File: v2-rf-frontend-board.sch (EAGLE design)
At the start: 150 parts, among them J1 1.27MM-SWD-CONNECTOR, J2 CON_SMA-ENDFIRE_EMERSON_EMERS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, J3 ROCKETNET-CONNECTOR-16M, J4 ZX62D-B-5P8, J5 BREAKOUT, J7 CON_HIROSE_DM3D(MICROSD), Q1 NTR4101P, T1 ALT4532, T2 ALT4532, U1 MAX2769, U2 STM32F4V_100PIN_GPSBOARD, U3 KSZ8081, U4 7Q-16.368MBG-T, U5 XC2401A8167R-G, U6 MAX8510EXK29+T, U7 MAX8510EXK29+T, U8 LMZ12001, X1 25 MHz

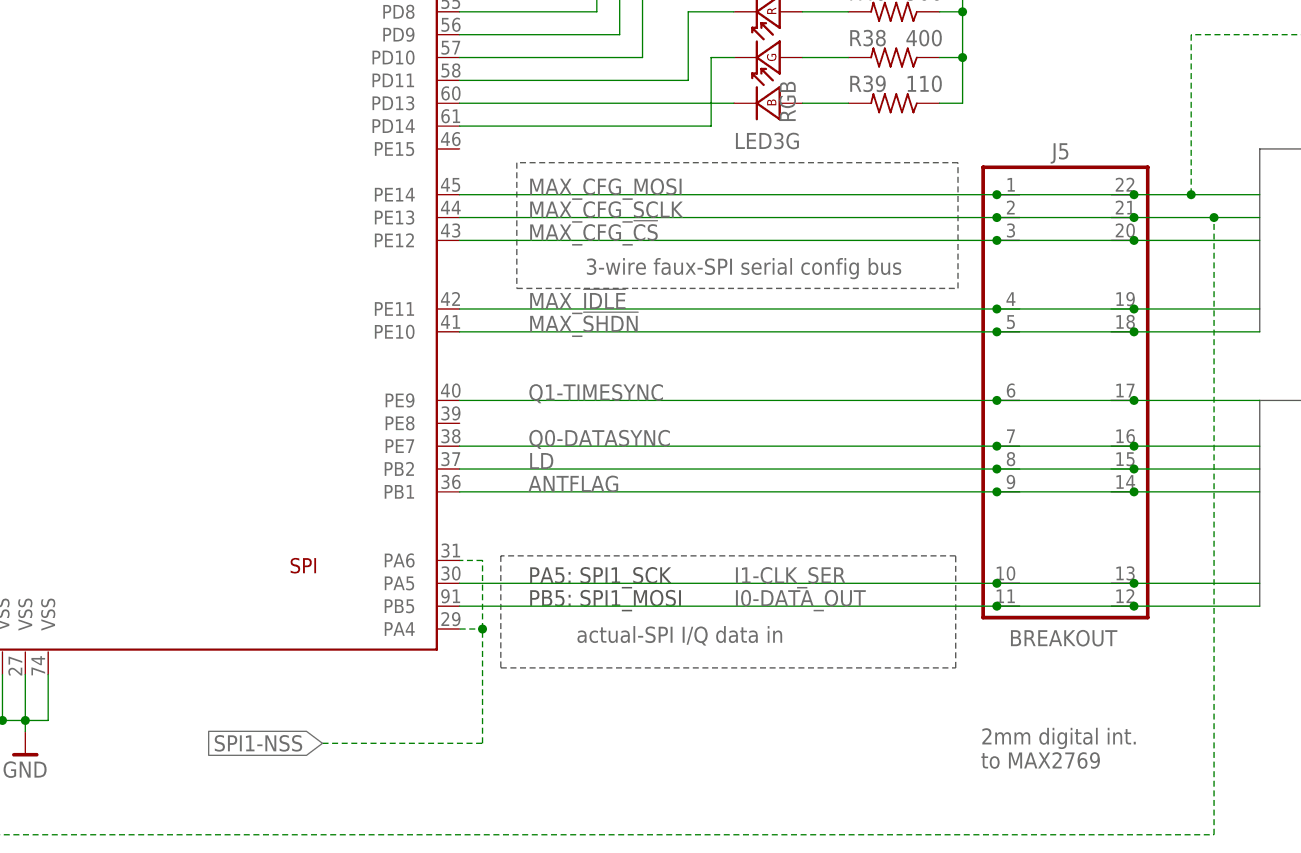
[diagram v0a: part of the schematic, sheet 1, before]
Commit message: Cleaned up modwire patches a bit. Added cuts in 0.1" double header.
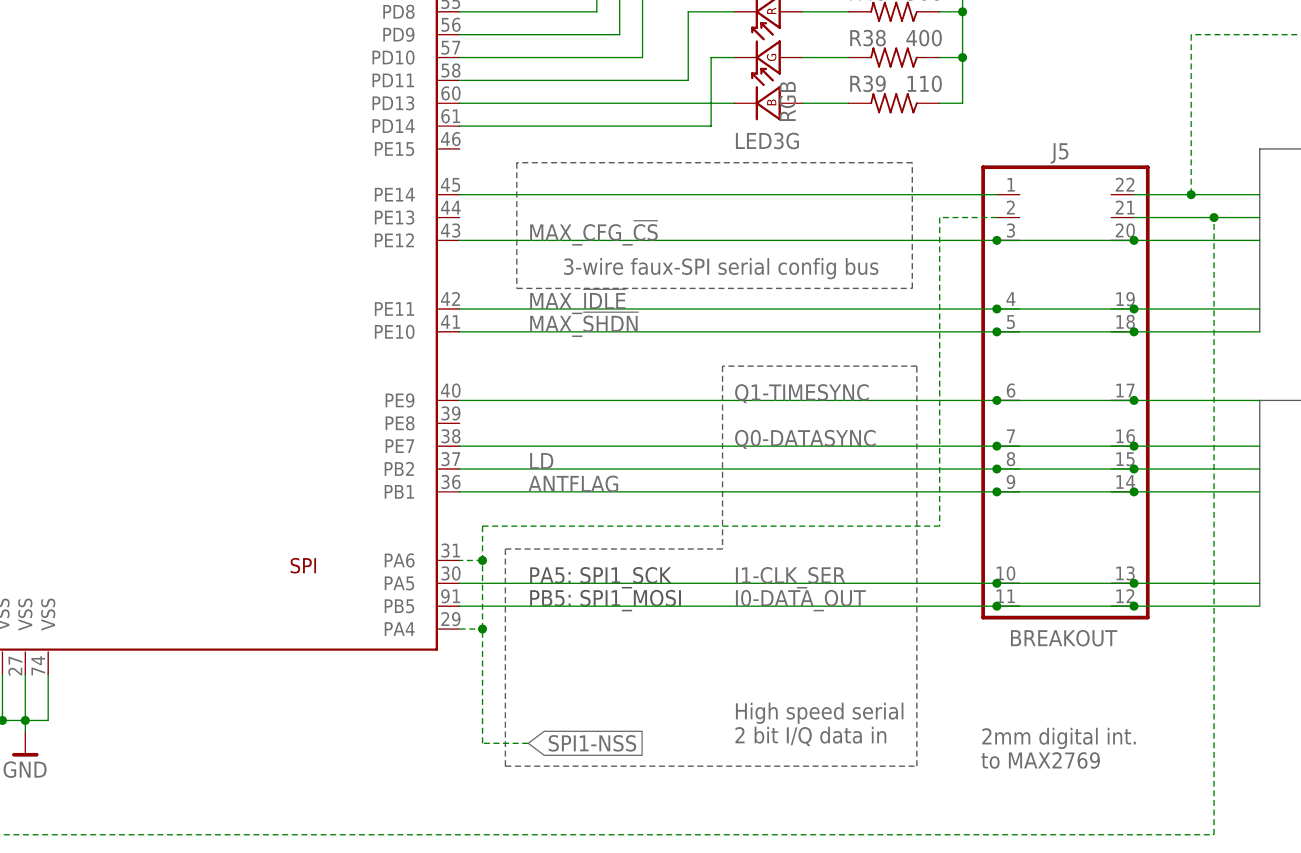
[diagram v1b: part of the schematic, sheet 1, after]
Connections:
- new net N$4: J5.1, U2.PE14
- net MAX_CFG_MOSI: no longer J5.1, U2.PE14
- net MAX_CFG_SCLK: no longer J5.2, U2.PE13
- net SPI1-NSS: now also J5.2
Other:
- note added: "High speed serial 2 bit I/Q data in"
- note removed: "actual-SPI I/Q data in"
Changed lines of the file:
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@@
 <?xml version="1.0" encoding="utf-8"?>
 <!DOCTYPE eagle SYSTEM "eagle.dtd">
-<eagle version="6.5.0">
+<eagle version="6.6.0">
 <drawing>
 <settings>
@@
 <setting verticaltext="up"/>
 </settings>
-<grid distance="0.1" unitdist="inch" unit="mm" style="lines" multiple="1" display="yes" altdistance="0.01" altunitdist="inch" altunit="mm"/>
+<grid distance="0.05" unitdist="inch" unit="inch" style="lines" multiple="2" display="yes" altdistance="0.01" altunitdist="inch" altunit="inch"/>
 <layers>
 <layer number="1" name="Top" color="4" fill="1" visible="no" active="no"/>
@@
 <description>STM</description>
 <plain>
-<text x="257.81" y="90.17" size="1.778" layer="95">3-wire faux-SPI serial config bus</text>
+<text x="255.27" y="90.17" size="1.778" layer="95">3-wire faux-SPI serial config bus</text>
 <text x="54.61" y="189.23" size="1.778" layer="97">NC</text>
 <text x="301.752" y="35.306" size="1.778" layer="95">2mm digital int.
 to MAX2769</text>
 <wire x1="250.19" y1="102.616" x2="250.19" y2="88.646" width="0.1524" layer="97" style="longdash"/>
-<wire x1="250.19" y1="88.646" x2="299.212" y2="88.646" width="0.1524" layer="97" style="longdash"/>
-<wire x1="299.212" y1="88.646" x2="299.212" y2="102.616" width="0.1524" layer="97" style="longdash"/>
-<wire x1="299.212" y1="102.616" x2="250.19" y2="102.616" width="0.1524" layer="97" style="longdash"/>
-<text x="256.794" y="49.276" size="1.778" layer="95">actual-SPI I/Q data in</text>
-<wire x1="248.412" y1="58.928" x2="248.412" y2="46.482" width="0.1524" layer="97" style="longdash"/>
-<wire x1="298.958" y1="58.928" x2="248.412" y2="58.928" width="0.1524" layer="97" style="longdash"/>
-<wire x1="298.958" y1="46.482" x2="298.958" y2="58.928" width="0.1524" layer="97" style="longdash"/>
-<wire x1="248.412" y1="46.482" x2="298.958" y2="46.482" width="0.1524" layer="97" style="longdash"/>
+<wire x1="250.19" y1="88.646" x2="294.132" y2="88.646" width="0.1524" layer="97" style="longdash"/>
+<wire x1="294.132" y1="88.646" x2="294.132" y2="102.616" width="0.1524" layer="97" style="longdash"/>
+<wire x1="294.132" y1="102.616" x2="250.19" y2="102.616" width="0.1524" layer="97" style="longdash"/>
+<text x="274.32" y="38.1" size="1.778" layer="95">High speed serial
+2 bit I/Q data in</text>
+<wire x1="248.92" y1="35.56" x2="294.64" y2="35.56" width="0.1524" layer="97" style="longdash"/>
+<wire x1="294.64" y1="35.56" x2="294.64" y2="80.01" width="0.1524" layer="97" style="longdash"/>
+<wire x1="294.64" y1="80.01" x2="273.05" y2="80.01" width="0.1524" layer="97" style="longdash"/>
+<wire x1="273.05" y1="80.01" x2="273.05" y2="59.69" width="0.1524" layer="97" style="longdash"/>
+<wire x1="273.05" y1="59.69" x2="248.92" y2="59.69" width="0.1524" layer="97" style="longdash"/>
+<wire x1="248.92" y1="59.69" x2="248.92" y2="35.56" width="0.1524" layer="97" style="longdash"/>
 <wire x1="35.56" y1="149.352" x2="35.56" y2="148.59" width="0.1524" layer="94"/>
 <wire x1="35.56" y1="148.59" x2="35.56" y2="102.616" width="0.4064" layer="94"/>
@@
 <text x="326.39" y="41.91" size="1.778" layer="102" rot="R90">MODWIRE</text>
 <text x="110.49" y="92.71" size="1.778" layer="102" rot="R90">MODWIRE</text>
-<text x="244.094" y="40.894" size="1.778" layer="102" rot="R180">MODWIRE</text>
+<text x="243.586" y="49.784" size="1.778" layer="102" rot="R270">MODWIRE</text>
 </plain>
 <instances>
@@
 <net name="MAX_CFG_MOSI" class="0">
 <segment>
-<label x="251.46" y="99.06" size="1.778" layer="95"/>
-<wire x1="303.53" y1="99.06" x2="243.84" y2="99.06" width="0.1524" layer="91"/>
-<pinref part="J5" gate="G$1" pin="1"/>
 <pinref part="J5" gate="G$1" pin="22"/>
-<wire x1="303.53" y1="99.06" x2="318.77" y2="99.06" width="0.1524" layer="91"/>
 <wire x1="318.77" y1="99.06" x2="325.12" y2="99.06" width="0.1524" layer="91"/>
-<junction x="318.77" y="99.06"/>
-<junction x="303.53" y="99.06"/>
-<pinref part="U2" gate="U" pin="PE14"/>
 <pinref part="U2" gate="U" pin="PB15"/>
 <wire x1="325.12" y1="99.06" x2="332.74" y2="99.06" width="0.1524" layer="91"/>
@@
 <pinref part="J5" gate="G$1" pin="21"/>
 <wire x1="318.77" y1="96.52" x2="327.66" y2="96.52" width="0.1524" layer="91"/>
-<label x="251.46" y="96.52" size="1.778" layer="95"/>
 <wire x1="327.66" y1="96.52" x2="332.74" y2="96.52" width="0.1524" layer="91"/>
-<wire x1="303.53" y1="96.52" x2="243.84" y2="96.52" width="0.1524" layer="91"/>
-<pinref part="J5" gate="G$1" pin="2"/>
-<wire x1="318.77" y1="96.52" x2="303.53" y2="96.52" width="0.1524" layer="91"/>
-<junction x="303.53" y="96.52"/>
-<junction x="318.77" y="96.52"/>
-<pinref part="U2" gate="U" pin="PE13"/>
 <pinref part="U2" gate="U" pin="PB10"/>
 <wire x1="160.02" y1="81.28" x2="147.32" y2="81.28" width="0.1524" layer="91" style="shortdash"/>
@@
 <net name="Q0-DATASYNC" class="0">
 <segment>
-<label x="251.46" y="71.12" size="1.778" layer="95"/>
+<label x="274.32" y="71.12" size="1.778" layer="95"/>
 <wire x1="303.53" y1="71.12" x2="243.84" y2="71.12" width="0.1524" layer="91"/>
 <pinref part="J5" gate="G$1" pin="7"/>
@@
 <net name="Q1-TIMESYNC" class="0">
 <segment>
-<label x="251.46" y="76.2" size="1.778" layer="95"/>
+<label x="274.32" y="76.2" size="1.778" layer="95"/>
 <wire x1="303.53" y1="76.2" x2="243.84" y2="76.2" width="0.1524" layer="91"/>
 <pinref part="J5" gate="G$1" pin="6"/>
@@
 <pinref part="U2" gate="U" pin="PA6"/>
 <wire x1="246.38" y1="58.42" x2="243.84" y2="58.42" width="0.1524" layer="91" style="shortdash"/>
-<label x="228.6" y="38.1" size="1.778" layer="102" rot="R180" xref="yes"/>
-<wire x1="228.6" y1="38.1" x2="246.38" y2="38.1" width="0.1524" layer="91" style="shortdash"/>
+<label x="251.46" y="38.1" size="1.778" layer="102" xref="yes"/>
+<wire x1="251.46" y1="38.1" x2="246.38" y2="38.1" width="0.1524" layer="91" style="shortdash"/>
 <wire x1="246.38" y1="38.1" x2="246.38" y2="50.8" width="0.1524" layer="91" style="shortdash"/>
 <junction x="246.38" y="50.8"/>
-</segment>
-</net>
+<wire x1="303.53" y1="96.52" x2="297.18" y2="96.52" width="0.1524" layer="91" style="shortdash"/>
+<wire x1="297.18" y1="96.52" x2="297.18" y2="62.23" width="0.1524" layer="91" style="shortdash"/>
+<wire x1="297.18" y1="62.23" x2="246.38" y2="62.23" width="0.1524" layer="91" style="shortdash"/>
+<wire x1="246.38" y1="62.23" x2="246.38" y2="58.42" width="0.1524" layer="91" style="shortdash"/>
+<junction x="246.38" y="58.42"/>
+<pinref part="J5" gate="G$1" pin="2"/>
+</segment>
+</net>
+<net name="N$4" class="0">
+<segment>
+<pinref part="J5" gate="G$1" pin="1"/>
+<wire x1="303.53" y1="99.06" x2="243.84" y2="99.06" width="0.1524" layer="91"/>
+<pinref part="U2" gate="U" pin="PE14"/>
+</segment>
+</net>
